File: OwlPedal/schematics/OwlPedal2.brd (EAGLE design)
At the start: 103.1 x 79.5 mm, 88 parts, among them IC1 7805TV, IC6 TS924, J1 NEUTRIK_NMJ6HCD2, J2 NEUTRIK_NMJ6HCD2, J3 NEUTRIK_NMJ6HCD2, J4 NEUTRIK_NMJ6HCD2, J5 NEUTRIK_NMJ6HCD2, J6 NEUTRIK_NMJ6HCD2, J7 POWER_JACK, T1 BC846, T2 2N7002P

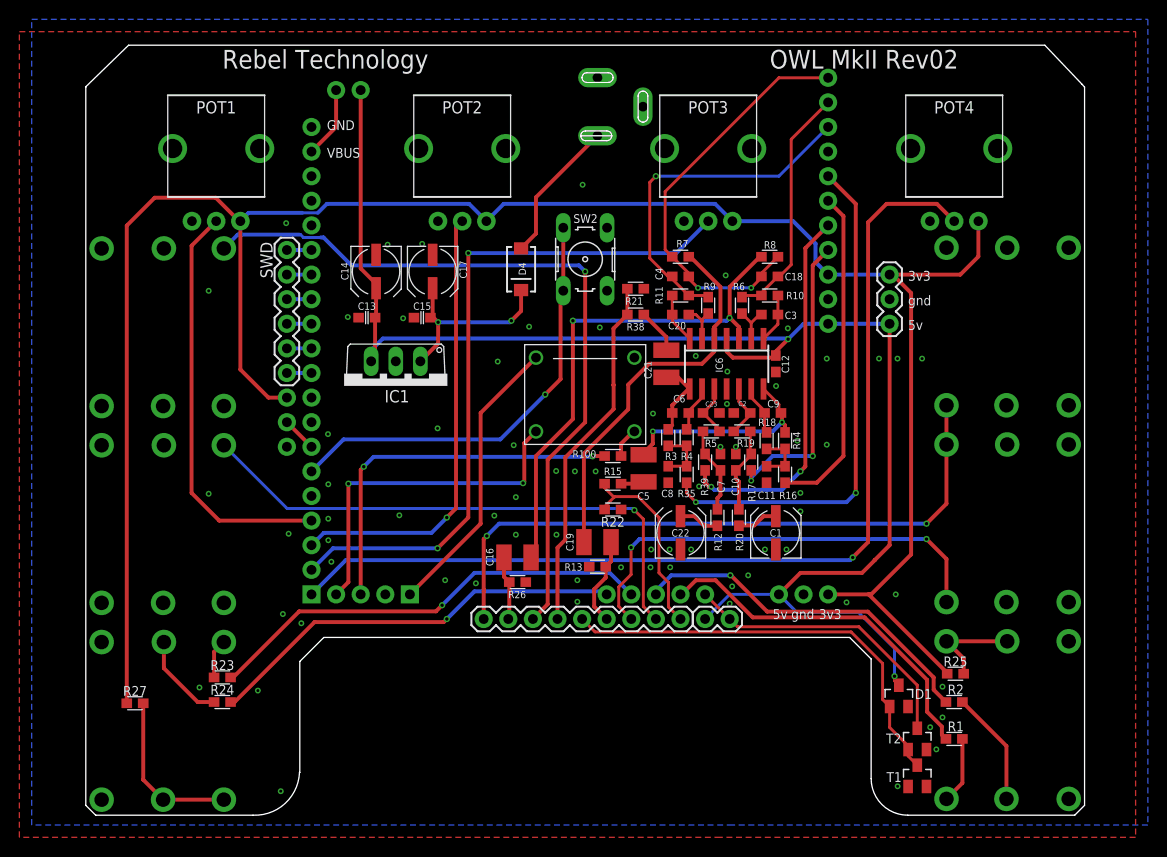
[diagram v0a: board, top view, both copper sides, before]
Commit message: Rev02
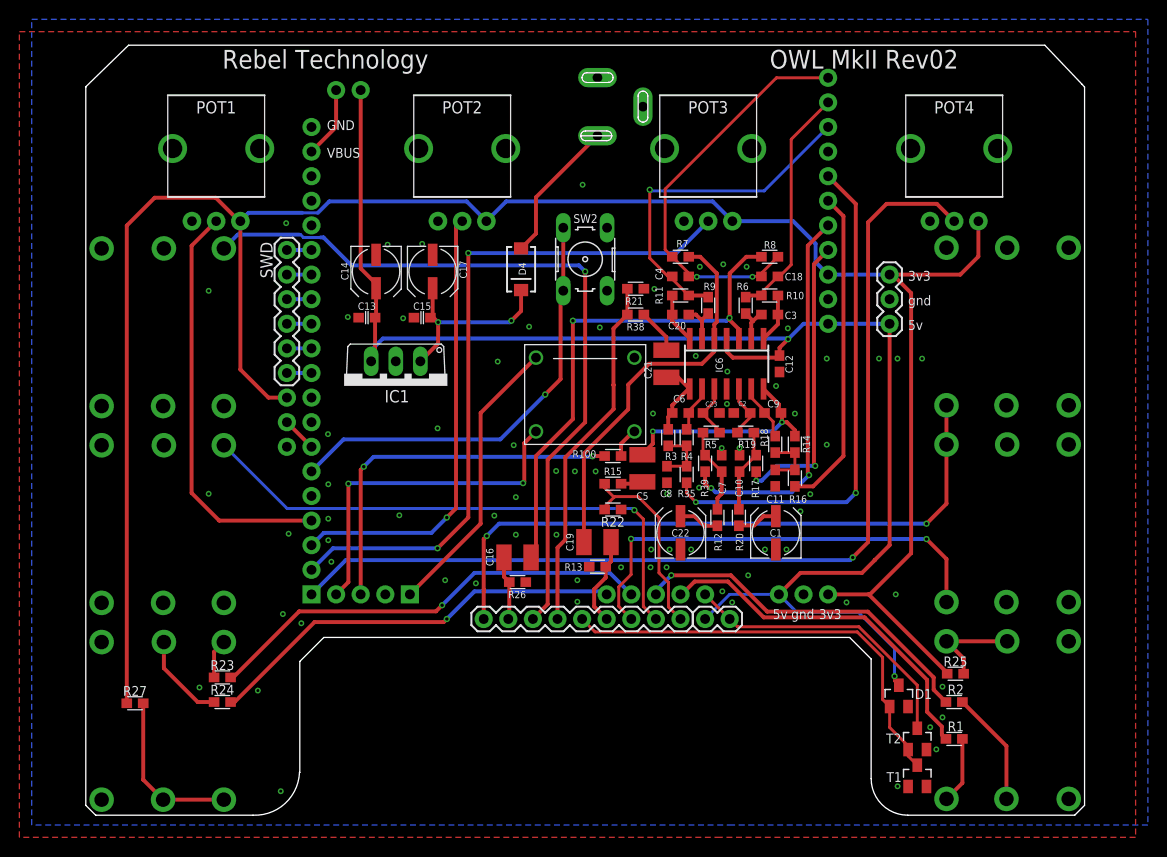
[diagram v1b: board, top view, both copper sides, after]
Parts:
- moved R14 1.09 mm to (72.5, 39.3)
- moved R16 1.09 mm to (72.5, 35.8)
- moved C11 0.97 mm to (70.4, 35.8)
- moved R18 0.97 mm to (70.4, 39.3)
- moved R17 0.52 mm to (68.5, 37.3)
- moved C10 0.40 mm to (66.7, 37.3)
- moved R19 0.40 mm to (67.4, 40.5)
- moved C12 0.38 mm to (70.9, 47.6)
- moved R6 0.38 mm to (67.4, 53.7)
- moved C7 0.18 mm to (64.9, 37.3)
- moved C5 0.13 mm to (56.7, 36.8)
- moved C8 0.13 mm to (59.2, 36.2)
- moved R39 0.13 mm to (63.2, 37.3)
- moved R5 0.13 mm to (63.8, 40.5)
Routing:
- net N$37: track 21.9 -> 23.1 mm
- net CS_VREF: track 42.9 -> 41.9 mm
- net AOUT_A+: track 38.8 -> 39.8 mm
- net AOUT_B-: track 34.2 -> 33.3 mm
- net DC_IN_L: track 52.9 -> 53.7 mm
- net N$19: track 5.45 -> 6.20 mm
- net IN_R: track 46.7 -> 47.2 mm
- net GND: track 1.48 -> 1.47 mm, vias 72 -> 76
